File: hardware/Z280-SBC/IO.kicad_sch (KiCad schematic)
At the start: 20 parts, among them J1 CompactFlash, J2 Serial1, J3 POWER, U1 74HC14, U6 74HC08, U9 74HC32

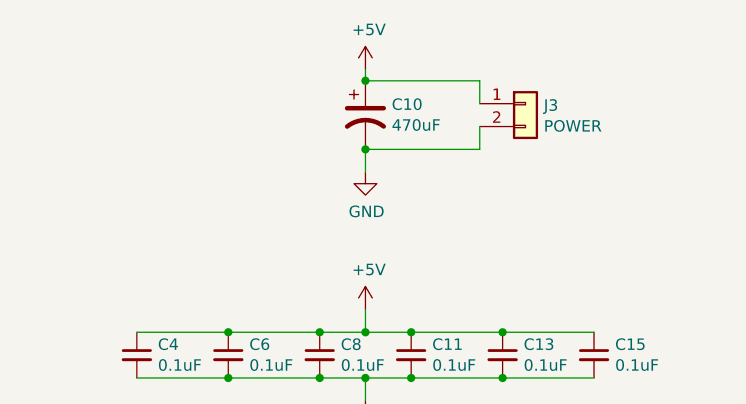
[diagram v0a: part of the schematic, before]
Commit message: Mostly done Rev1
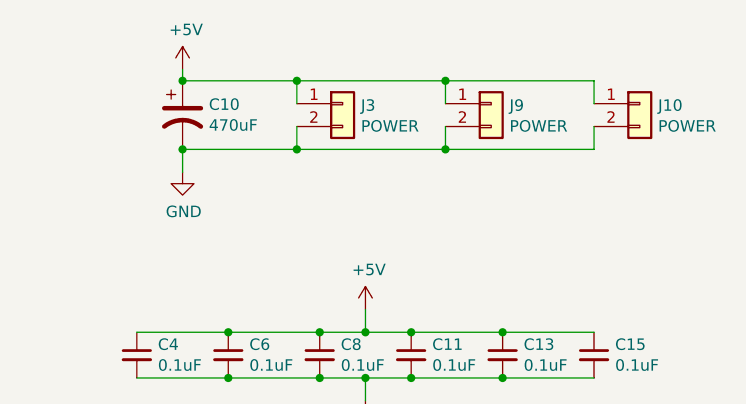
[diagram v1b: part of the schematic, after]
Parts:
- added J10, J9: POWER, Connector_PinHeader_2.54mm:PinHeader_1x02_P2.54mm_Vertical, symbol Connector_Generic:Conn_01x02
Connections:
- net +5V: now also J10.1 (Pin_1), J9.1 (Pin_1)
- net GND: now also J10.2 (Pin_2), J9.2 (Pin_2)
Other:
- moved on the sheet: C10, J3
